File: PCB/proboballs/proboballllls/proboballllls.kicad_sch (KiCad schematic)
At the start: 1 part, among them J1 Conn_01x22_Socket

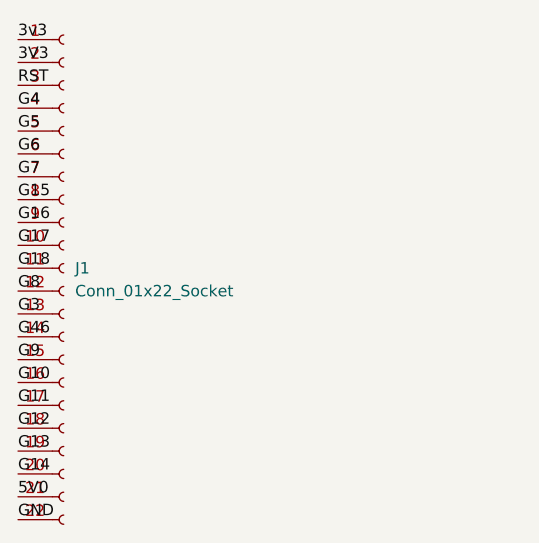
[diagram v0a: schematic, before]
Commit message: new balls
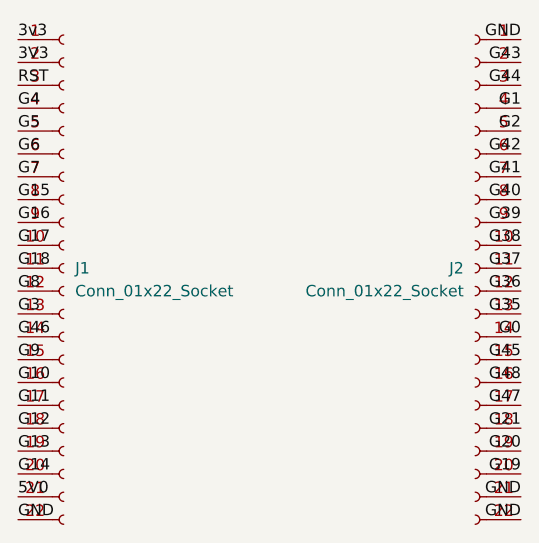
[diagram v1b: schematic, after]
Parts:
- added J2: Conn_01x22_Socket, symbol Connector:Conn_01x22_Socket
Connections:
- net GND: now also J2.1 (Pin_1), J2.21 (Pin_21), J2.22 (Pin_22)
- new net G0: J2.14 (Pin_14)
- new net G1: J2.4 (Pin_4)
- new net G19: J2.20 (Pin_20)
- new net G2: J2.5 (Pin_5)
- new net G20: J2.19 (Pin_19)
- new net G21: J2.18 (Pin_18)
- new net G35: J2.13 (Pin_13)
- new net G36: J2.12 (Pin_12)
- new net G37: J2.11 (Pin_11)
- new net G38: J2.10 (Pin_10)
- new net G39: J2.9 (Pin_9)
- new net G40: J2.8 (Pin_8)
- new net G41: J2.7 (Pin_7)
- new net G42: J2.6 (Pin_6)
- new net G43: J2.2 (Pin_2)
- new net G44: J2.3 (Pin_3)
- new net G45: J2.15 (Pin_15)
- new net G47: J2.17 (Pin_17)
- new net G48: J2.16 (Pin_16)
